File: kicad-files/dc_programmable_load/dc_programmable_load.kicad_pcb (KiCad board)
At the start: 2 copper layers, 14 parts, among them J1 DC Jack 12V, J2 Conn_01x03_Socket, Q1 IRF3205, U2 LM317_SOT-223, U4 LM358DR

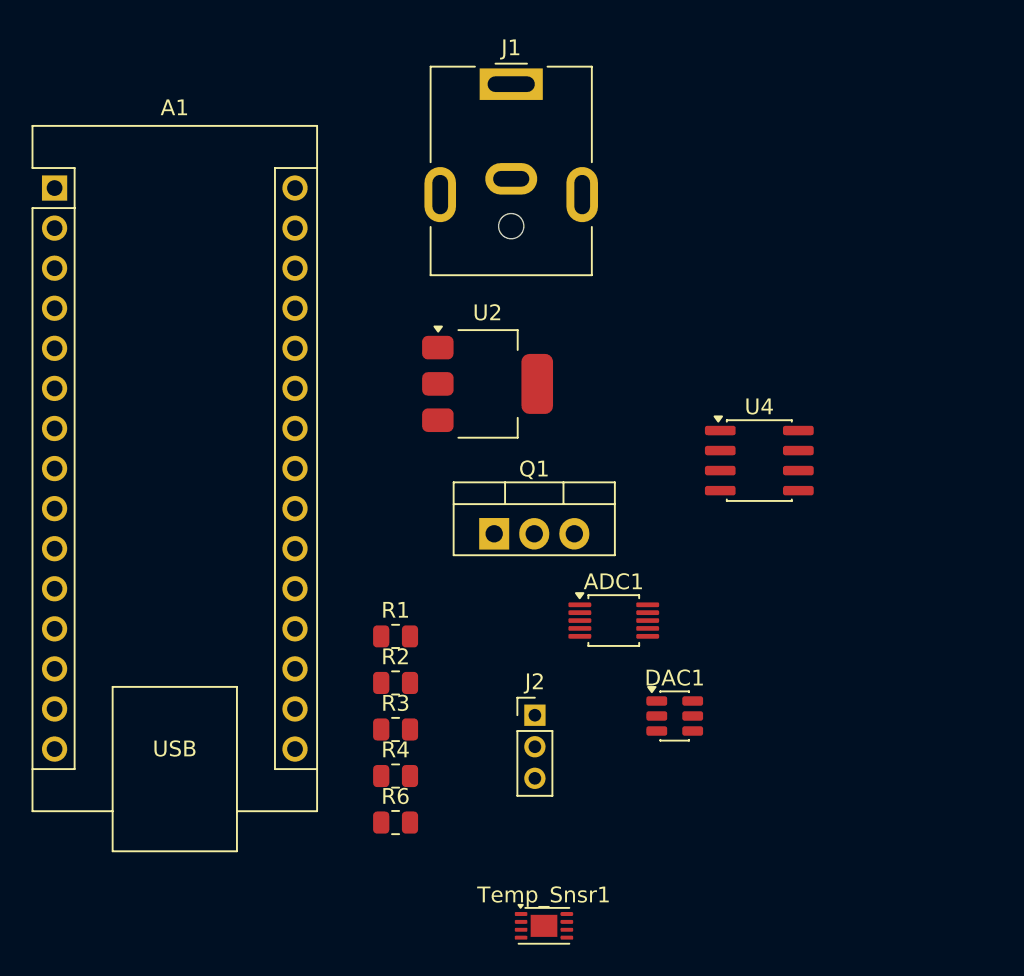
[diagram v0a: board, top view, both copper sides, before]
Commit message: version 1 of the PCB
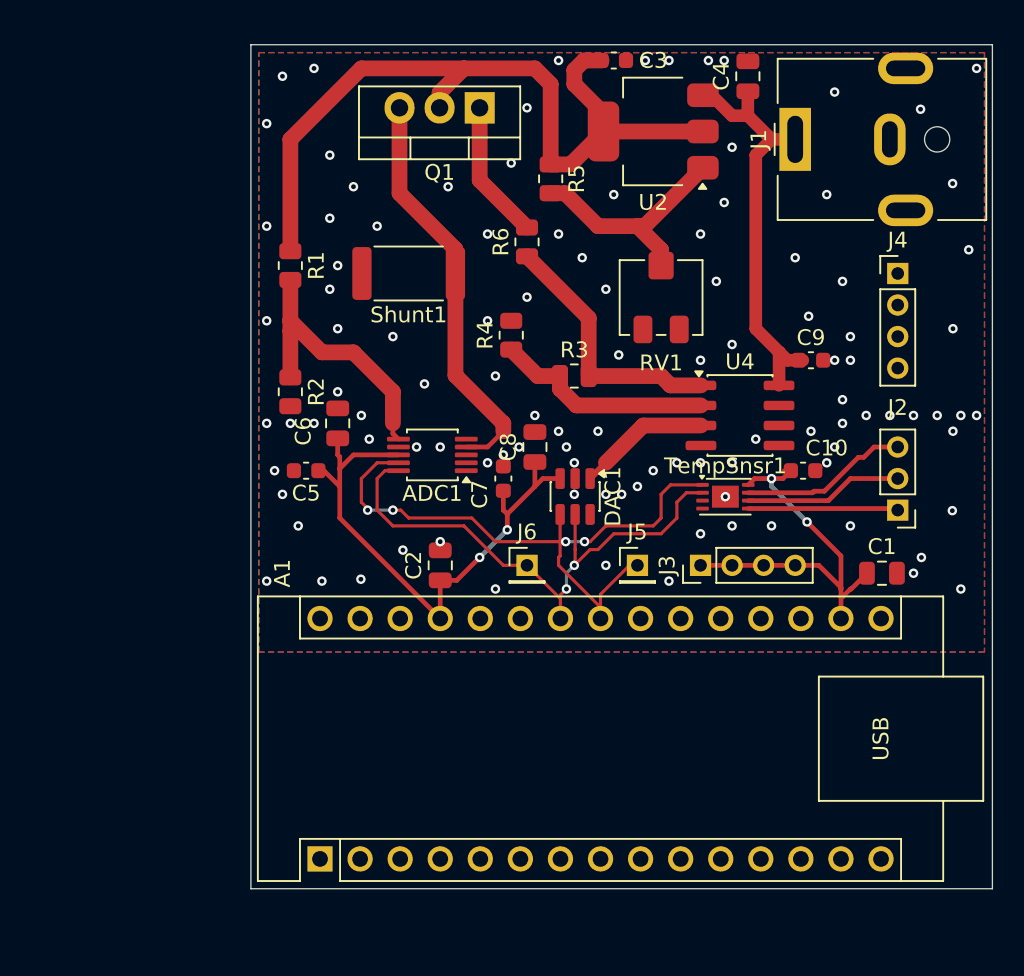
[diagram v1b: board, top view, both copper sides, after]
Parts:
- added C1: 10uF, Capacitor_SMD:C_0805_2012Metric, F.Cu at (166.0, 99.0)
- added C10: 100nF, Capacitor_SMD:C_0603_1608Metric, F.Cu at (161.0, 92.5)
- added C2: 10uF, Capacitor_SMD:C_0805_2012Metric, F.Cu at (138.0, 98.5)
- added C3: 100nF, Capacitor_SMD:C_0603_1608Metric, F.Cu at (149.0, 66.5)
- added C4: 10uF, Capacitor_SMD:C_0805_2012Metric, F.Cu at (157.5, 67.5)
- added C5: 100nF, Capacitor_SMD:C_0603_1608Metric, F.Cu at (129.5, 92.5)
- added C6: 1uF, Capacitor_SMD:C_0805_2012Metric, F.Cu at (131.5, 89.5)
- added C7: 100nF, Capacitor_SMD:C_0603_1608Metric, F.Cu at (142.0, 93.0)
- added C8: 1uF, Capacitor_SMD:C_0805_2012Metric, F.Cu at (144.0, 91.0)
- added C9: 100nF, Capacitor_SMD:C_0603_1608Metric, F.Cu at (161.5, 85.5)
- added J3: Conn_01x04_Socket, Connector_PinHeader_2.00mm:PinHeader_1x04_P2.00mm_Vertical, F.Cu at (154.5, 98.5)
- added J4: Conn_01x04_Socket, Connector_PinHeader_2.00mm:PinHeader_1x04_P2.00mm_Vertical, F.Cu at (167.0, 80.0)
- added J5: Conn_01x01_Socket, Connector_PinHeader_2.00mm:PinHeader_1x01_P2.00mm_Vertical, F.Cu at (150.5, 98.5)
- added J6: Conn_01x01_Socket, Connector_PinHeader_2.00mm:PinHeader_1x01_P2.00mm_Vertical, F.Cu at (143.5, 98.5)
- added R5: 10k, Resistor_SMD:R_0805_2012Metric, F.Cu at (145.0, 74.0)
- added RV1: R_Potentiometer, Potentiometer_SMD:Potentiometer_Bourns_3314S_Horizontal, F.Cu at (152.0, 81.5)
- added Shunt1: 1, Resistor_SMD:R_2512_6332Metric, F.Cu at (136.0, 80.0)
- moved A1 45.7 mm to (130.4, 117.1), turned to 90 degrees
- moved R6 37.7 mm to (143.5, 78.0), turned to 90 degrees
- moved TempSnsr1 29.5 mm to (156.1, 94.2)
- moved R4 28.9 mm to (142.5, 83.9), turned to 90 degrees
- moved Q1 27.0 mm to (140.5, 69.5), turned to 180 degrees
- moved J2 26.4 mm to (167.0, 95.0), turned to 180 degrees
- moved R3 25.1 mm to (146.5, 86.5)
- moved R1 24.4 mm to (128.5, 79.5), turned to -90 degrees
- moved R2 19.6 mm to (128.5, 87.5), turned to -90 degrees
- moved U2 19.1 mm to (151.5, 71.0), turned to 180 degrees
- moved J1 18.3 mm to (160.5, 71.5), turned to 90 degrees
- moved ADC1 15.6 mm to (137.5, 91.5), turned to 180 degrees
- moved DAC1 15.3 mm to (146.6, 94.1), turned to -90 degrees
- moved U4 3.11 mm to (157.0, 89.0)
- renumbered Temp_Snsr1 to TempSnsr1
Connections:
- net +5V renamed /Power Supply
- U2 pad 1: unconnected-(U2-ADJ-Pad1) -> Net-(U2-ADJ)
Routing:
- net /Power Supply: track 0.00 -> 51.7 mm
- net /sda: track 0.00 -> 41.9 mm, vias 0 -> 4
- net /5V: track 0.00 -> 36.4 mm, vias 0 -> 2
- net /scl: track 0.00 -> 36.4 mm, vias 0 -> 2
- net /12V: track 0.00 -> 26.4 mm
- net /3v3: track 0.00 -> 26.0 mm, vias 0 -> 2
- net /A0: track 0.00 -> 26.0 mm
- net /A2: track 0.00 -> 17.7 mm
- net /opamp_output: track 0.00 -> 16.6 mm
- net Net-(U2-ADJ): track 0.00 -> 15.2 mm
- net Net-(U4-1IN-): track 0.00 -> 14.0 mm
- net Net-(J2-Pin_3): track 0.00 -> 10.7 mm
- net Net-(J2-Pin_2): track 0.00 -> 10.1 mm
- net Net-(J2-Pin_1): track 0.00 -> 9.52 mm
- net Net-(Q1-G): track 0.00 -> 8.83 mm
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- added copper zone on B.Cu, net GND
- added copper zone on F.Cu, net GND
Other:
- board outline added: 47 x 53.5 mm
